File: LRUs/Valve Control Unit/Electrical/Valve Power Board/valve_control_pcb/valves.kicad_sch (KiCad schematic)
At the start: 6 parts

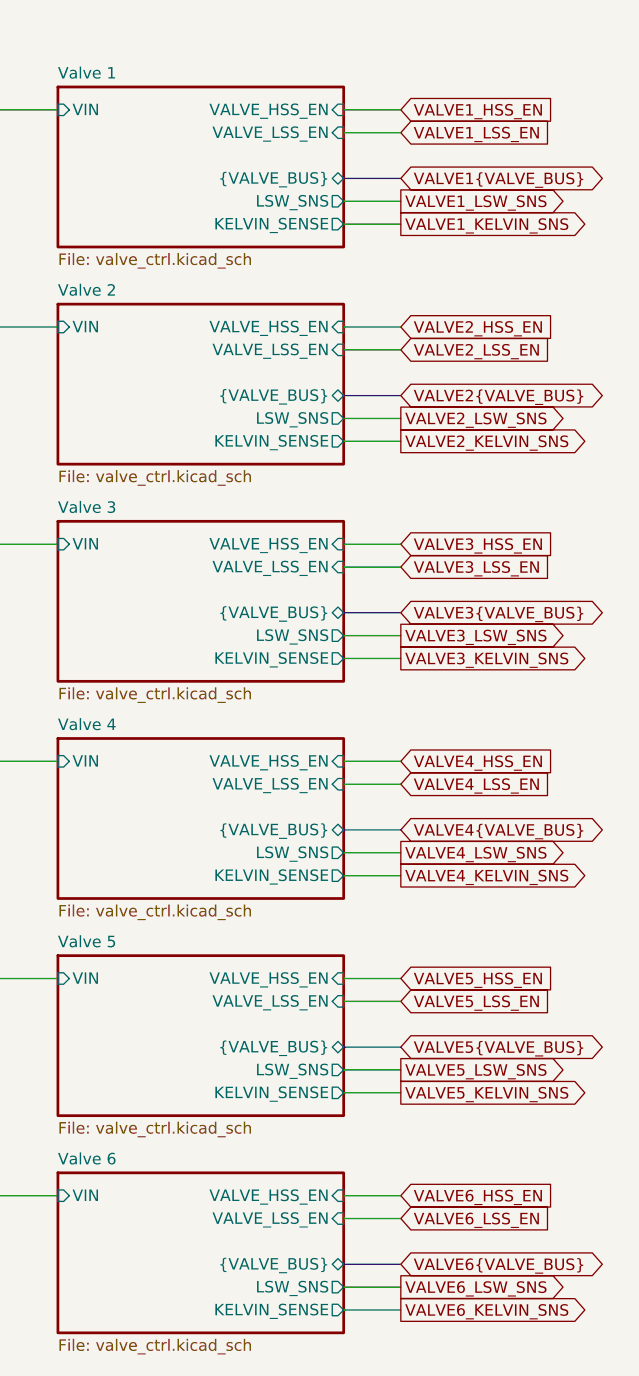
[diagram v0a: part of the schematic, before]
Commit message: Committttt
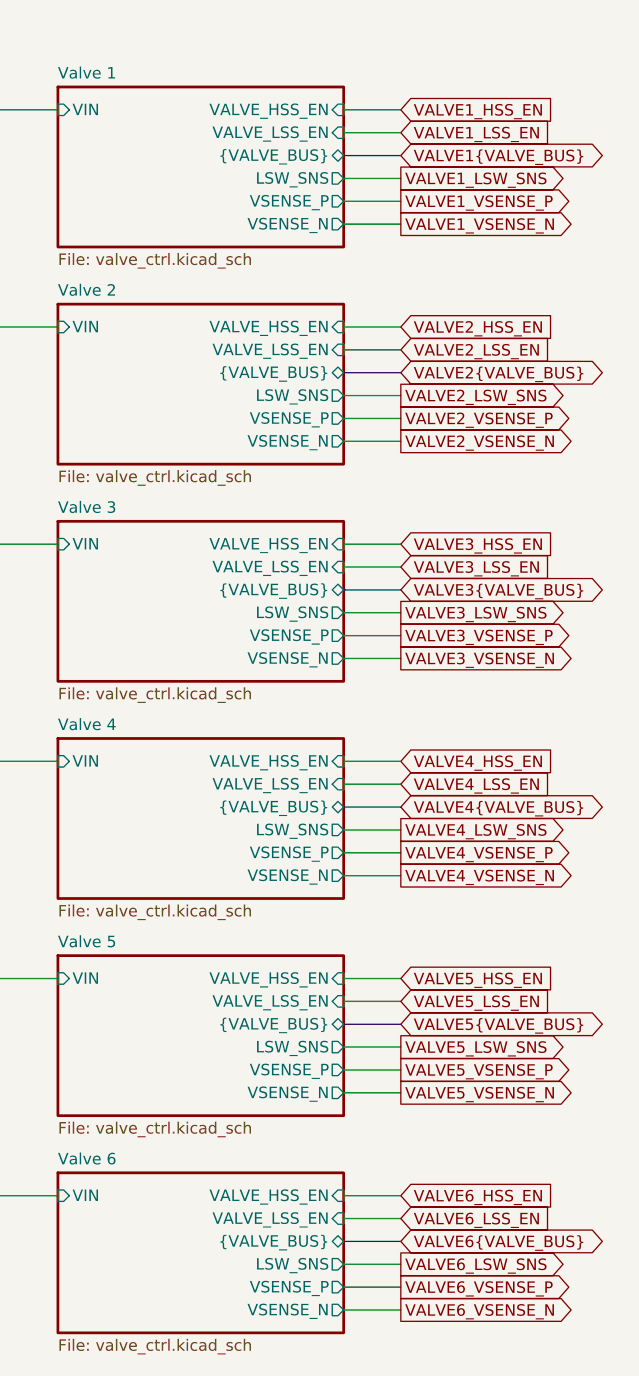
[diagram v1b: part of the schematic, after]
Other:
- sheet Valve 1 ports: added VSENSE_N, VSENSE_P; removed KELVIN_SENSE
- sheet Valve 2 ports: added VSENSE_N, VSENSE_P; removed KELVIN_SENSE
- sheet Valve 3 ports: added VSENSE_N, VSENSE_P; removed KELVIN_SENSE
- sheet Valve 4 ports: added VSENSE_N, VSENSE_P; removed KELVIN_SENSE
- sheet Valve 5 ports: added VSENSE_N, VSENSE_P; removed KELVIN_SENSE
- sheet Valve 6 ports: added VSENSE_N, VSENSE_P; removed KELVIN_SENSE
